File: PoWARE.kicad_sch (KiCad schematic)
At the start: 37 parts, among them J1 Conn_02x03_Counter_Clockwise, J2 Conn_02x03_Counter_Clockwise, J3 Screw_Terminal_01x02, J4 Conn_02x01, J5 Conn_02x01, J6 Conn_02x01, J7 Conn_02x01, P1 USB_C_Plug_USB2.0, SW1 SW_SPDT, SW2 SW_SP4T, U1 SY8303AIC, U2 CH224K

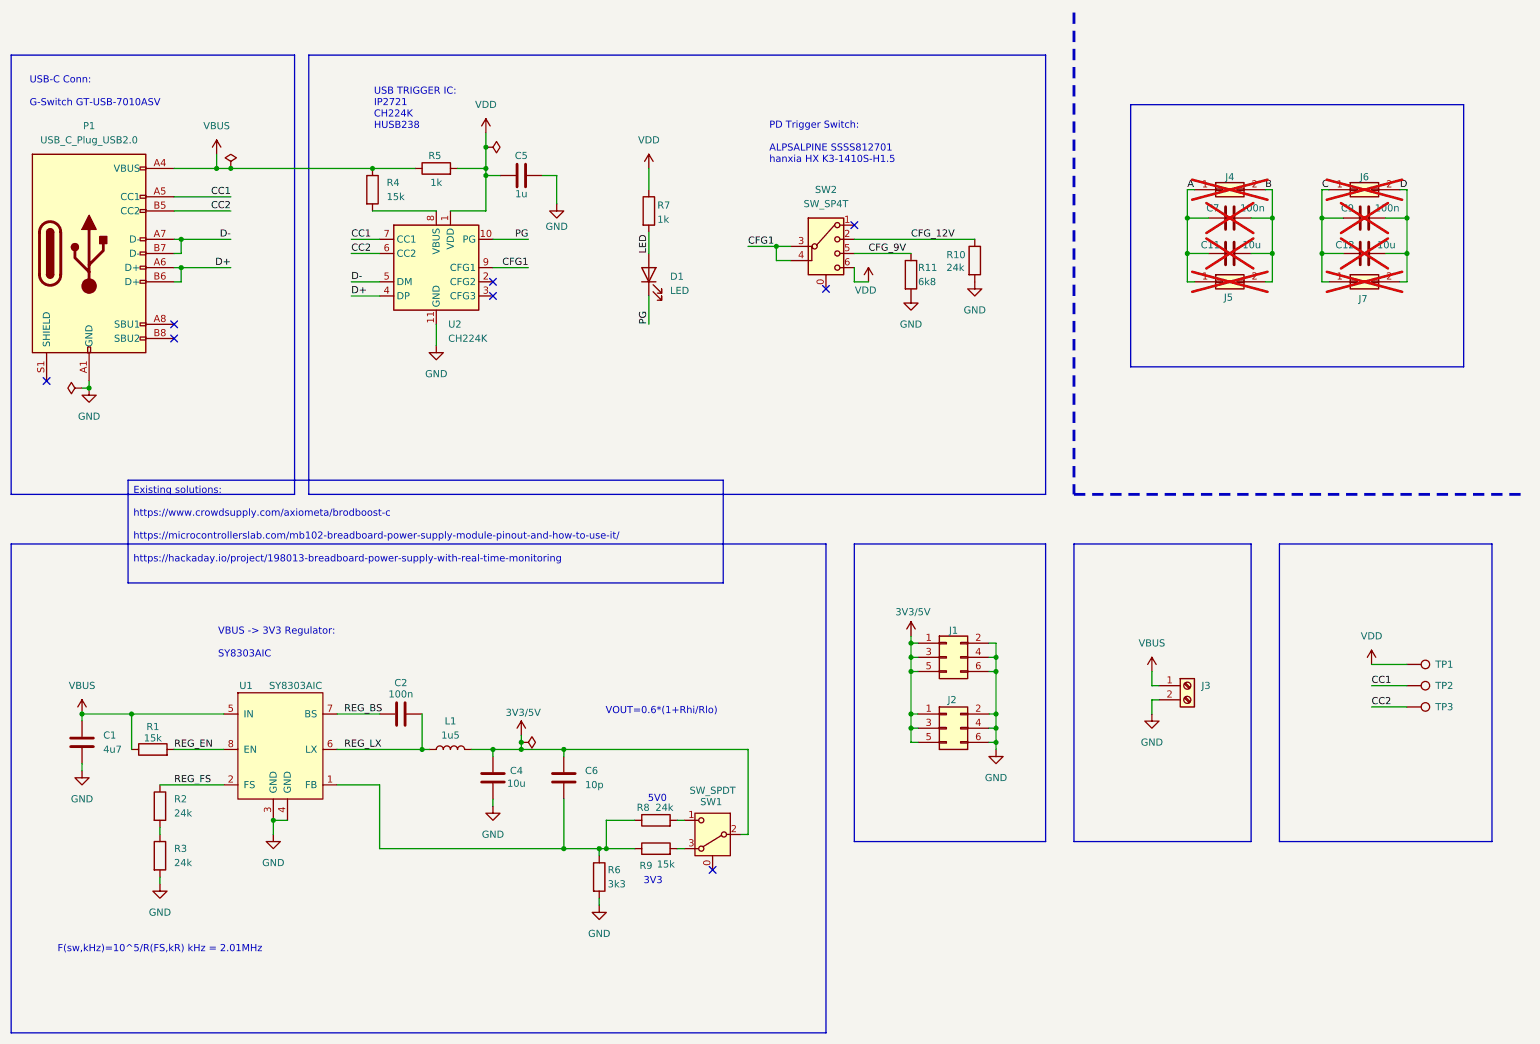
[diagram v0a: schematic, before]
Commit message: Cleaned up repo
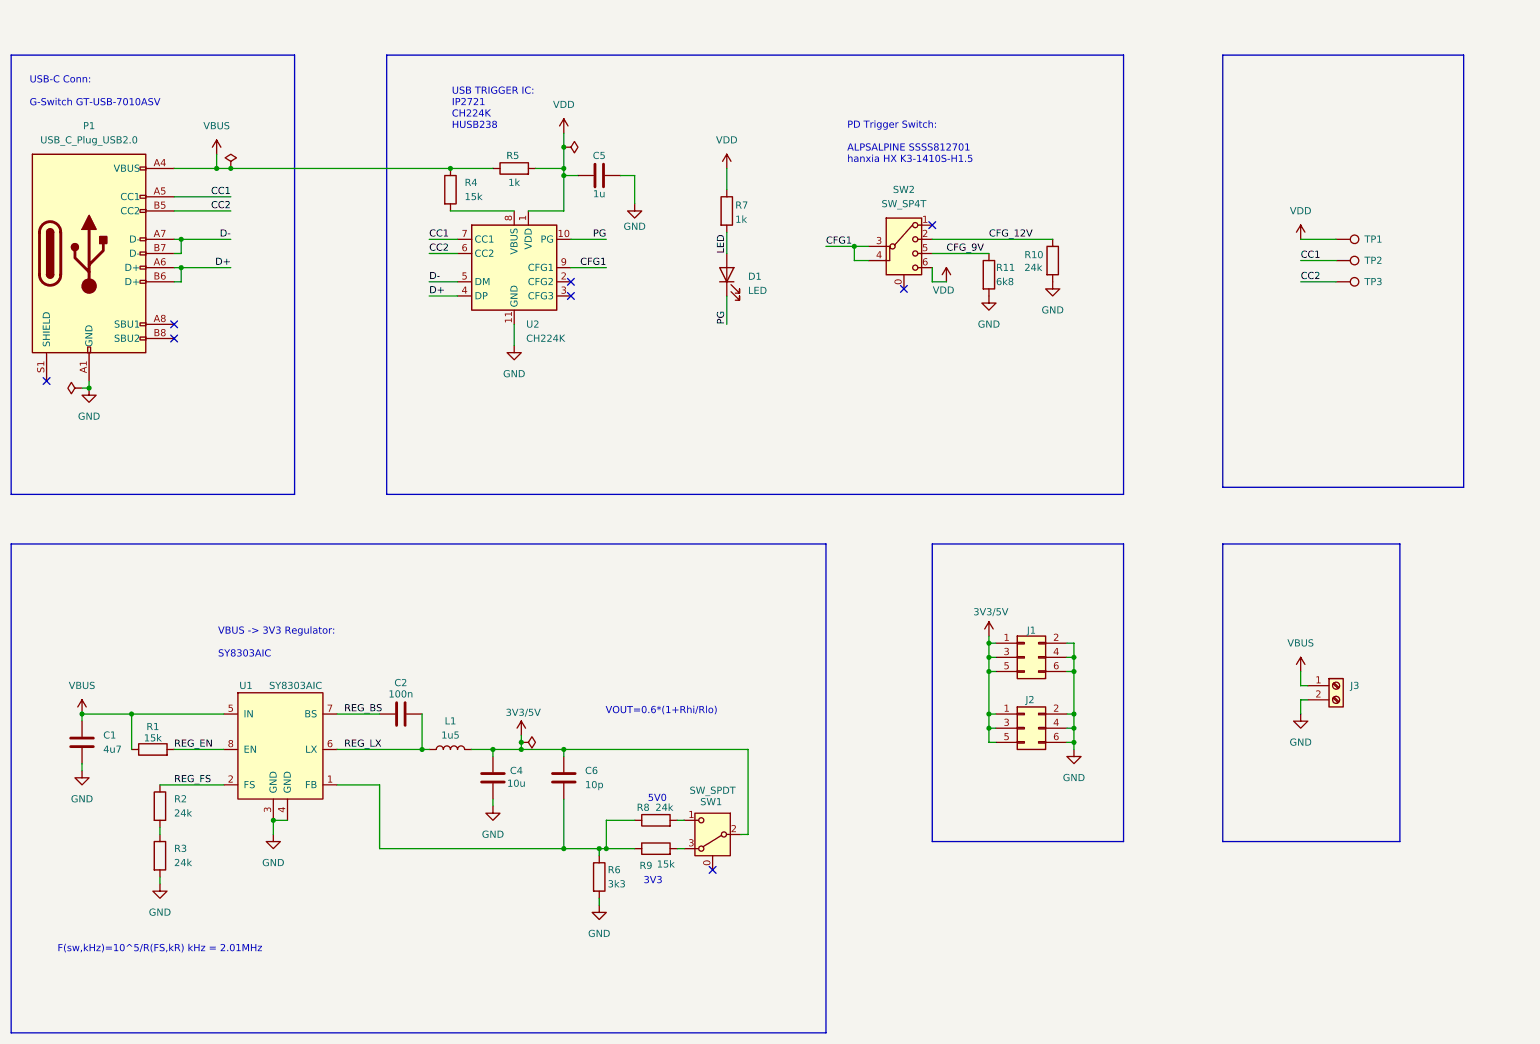
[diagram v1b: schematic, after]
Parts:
- removed C11, C12: 10u, Capacitor_SMD:C_0805_2012Metric, symbol Device:C
- removed C7, C9: 100n, Capacitor_SMD:C_0603_1608Metric, symbol Device:C
- removed J4, J5, J6, J7: Conn_02x01, Connector_PinHeader_2.54mm:PinHeader_2x01_P2.54mm_Vertical, symbol Connector_Generic:Conn_02x01
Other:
- moved on the sheet: C5, D1, J1, J2, J3, R10, R11, R4, R5, R7, SW2, TP1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
